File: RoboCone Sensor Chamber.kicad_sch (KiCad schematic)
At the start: 15 parts, among them J7 691210910002, U1 ADS1234IPW

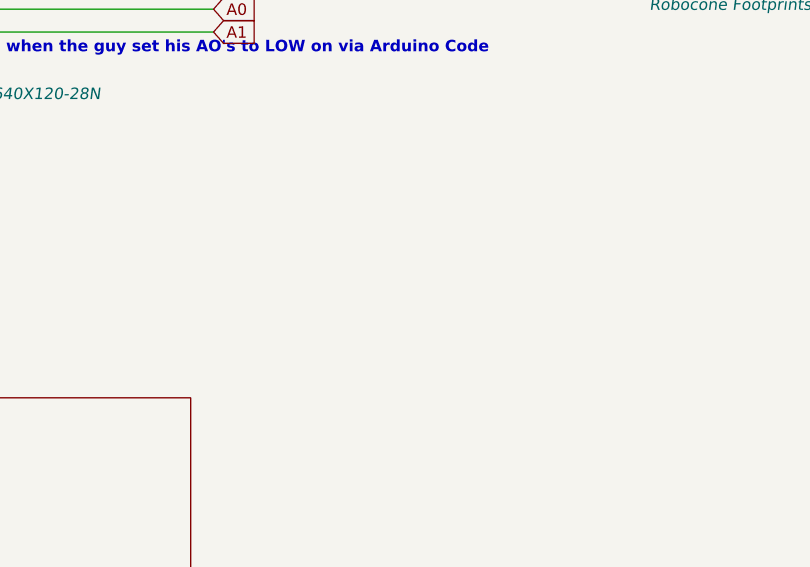
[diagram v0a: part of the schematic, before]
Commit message: test only
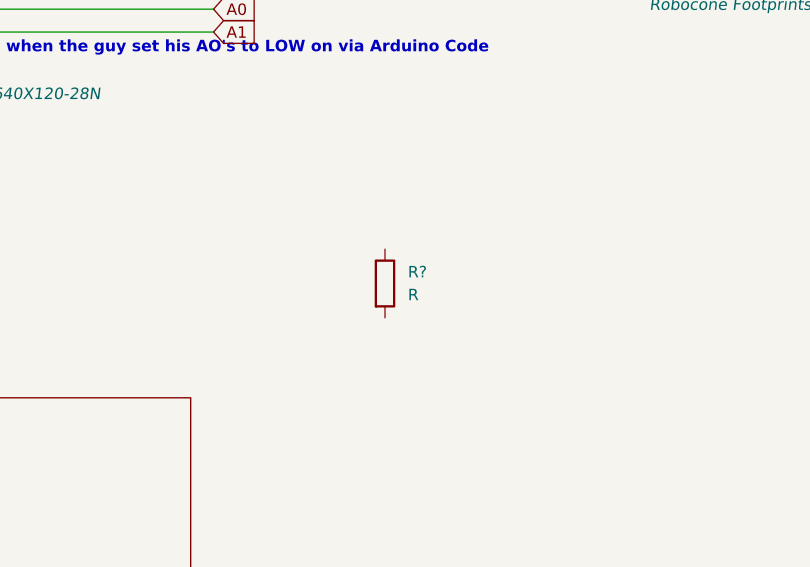
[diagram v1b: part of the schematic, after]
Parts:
- added R?: R, symbol Device:R
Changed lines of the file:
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@@
+	)
+	(symbol
+		(lib_id "Device:R")
+		(at 176.53 133.35 0)
+		(unit 1)
+		(exclude_from_sim no)
+		(in_bom yes)
+		(on_board yes)
+		(dnp no)
+		(fields_autoplaced yes)
+		(property "Reference" "R?"
+			(at 179.07 132.0799 0)
+			(effects
+				(font
+					(size 1.27 1.27)
+				)
+				(justify left)
+			)
+		)
+		(property "Value" "R"
+			(at 179.07 134.6199 0)
+			(effects
+				(font
+					(size 1.27 1.27)
+				)
+				(justify left)
+			)
+		)
+		(property "Footprint" ""
+			(at 174.752 133.35 90)
+			(effects
+				(font
+					(size 1.27 1.27)
+				)
+				(hide yes)
+			)
+		)
+		(property "Datasheet" "~"
+			(at 176.53 133.35 0)
+			(effects
+				(font
+					(size 1.27 1.27)
+				)
+				(hide yes)
+			)
+		)
+		(property "Description" "Resistor"
+			(at 176.53 133.35 0)
+			(effects
+				(font
+					(size 1.27 1.27)
+				)
+				(hide yes)
+			)
+		)
+		(pin "1"
+		)
+		(pin "2"
+		)
+		(instances
+			(project ""
+				(path "/4cbd4305-2804-444f-9b01-a0e20ec81091"
+					(reference "R?")
+					(unit 1)
+				)
+			)
+		)
 	)
 	(symbol

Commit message: back to normal now from test
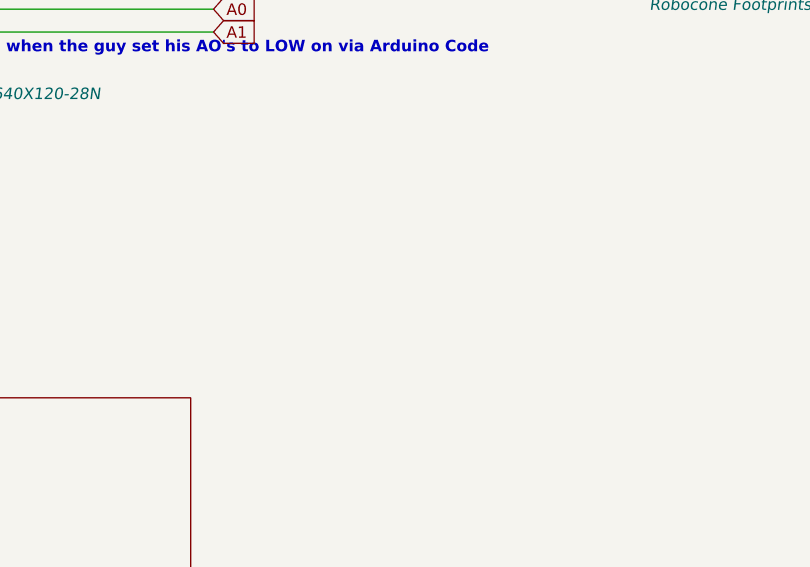
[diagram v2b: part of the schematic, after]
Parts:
- removed R?: R, symbol Device:R
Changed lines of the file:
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@@
-	)
-	(symbol
-		(lib_id "Device:R")
-		(at 176.53 133.35 0)
-		(unit 1)
-		(exclude_from_sim no)
-		(in_bom yes)
-		(on_board yes)
-		(dnp no)
-		(fields_autoplaced yes)
-		(property "Reference" "R?"
-			(at 179.07 132.0799 0)
-			(effects
-				(font
-					(size 1.27 1.27)
-				)
-				(justify left)
-			)
-		)
-		(property "Value" "R"
-			(at 179.07 134.6199 0)
-			(effects
-				(font
-					(size 1.27 1.27)
-				)
-				(justify left)
-			)
-		)
-		(property "Footprint" ""
-			(at 174.752 133.35 90)
-			(effects
-				(font
-					(size 1.27 1.27)
-				)
-				(hide yes)
-			)
-		)
-		(property "Datasheet" "~"
-			(at 176.53 133.35 0)
-			(effects
-				(font
-					(size 1.27 1.27)
-				)
-				(hide yes)
-			)
-		)
-		(property "Description" "Resistor"
-			(at 176.53 133.35 0)
-			(effects
-				(font
-					(size 1.27 1.27)
-				)
-				(hide yes)
-			)
-		)
-		(pin "1"
-		)
-		(pin "2"
-		)
-		(instances
-			(project ""
-				(path "/4cbd4305-2804-444f-9b01-a0e20ec81091"
-					(reference "R?")
-					(unit 1)
-				)
-			)
-		)
 	)
 	(symbol
